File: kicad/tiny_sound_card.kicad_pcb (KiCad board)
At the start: 2 copper layers, 46 parts, among them CON1 BARREL_JACK, IC1 ATMEGA328P-A, J1 TRS_JACK, M1 DFR0299, P1 EXT_PWR, P2 SPKOUT, P3 EXT_SW0, P4 EXT_I2C, P4 M3Drill, P5 EXT_SW1, P6 EXT_UART, P7 EXT_SPI/ISP, SW1 SlideSW, SW2 SW_PUSH, SW3 SW_PUSH, SW4 SW_PUSH, SW5 SlideSW, SW6 SW_PUSH, U1 STMPS2141S, Y1 16MHz

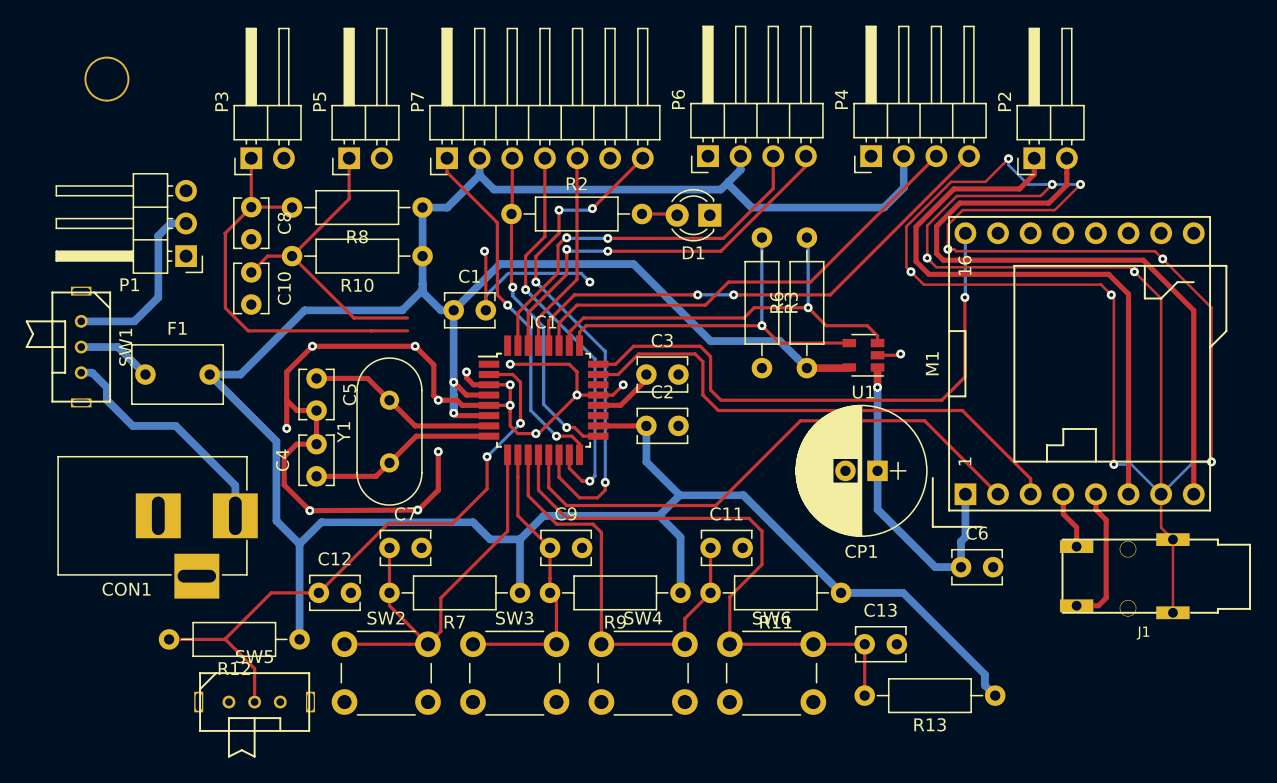
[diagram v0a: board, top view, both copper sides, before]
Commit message: 外形とパネル表裏を作成
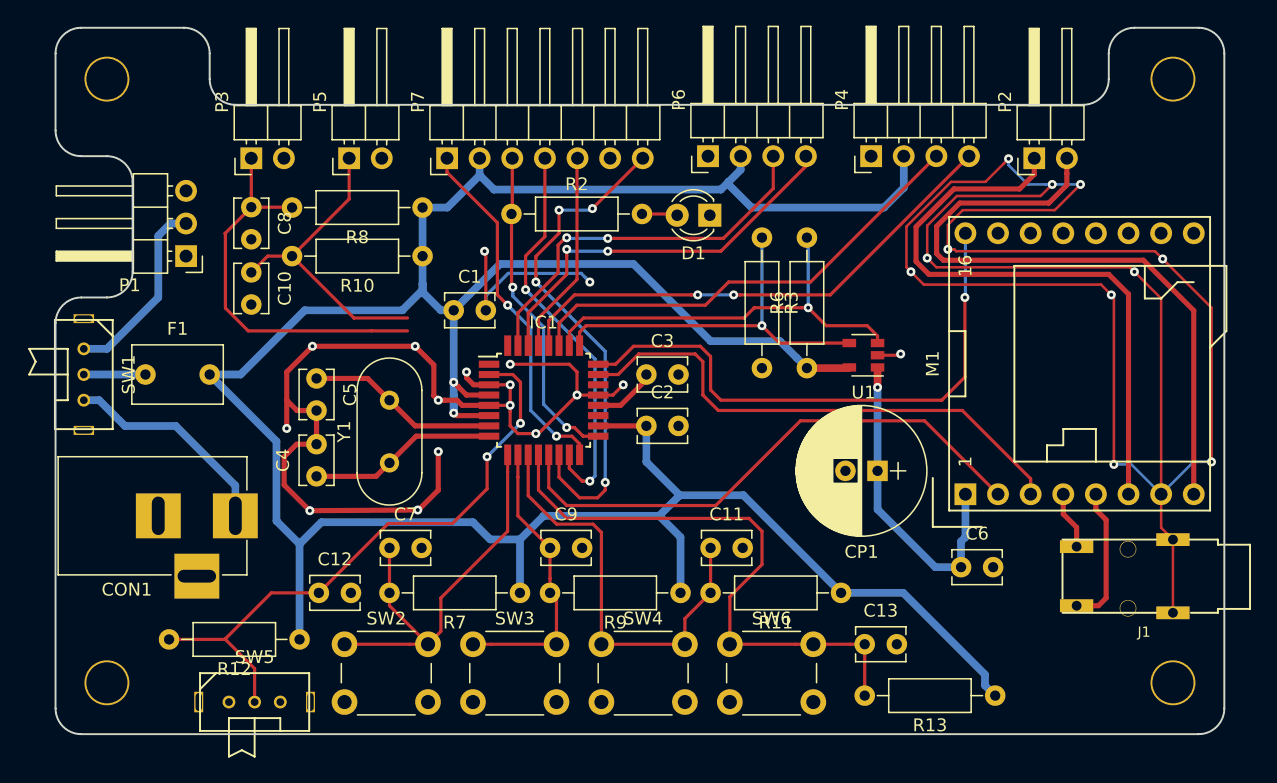
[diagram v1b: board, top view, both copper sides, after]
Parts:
- added P10: M3Drill, kamiya:M3Drill2, F.Cu at (138.0, 112.0)
- added P8: M3Drill, kamiya:M3Drill2, F.Cu at (55.0, 112.0)
- added P9: M3Drill, kamiya:M3Drill2, F.Cu at (138.0, 65.0)
- moved SW1 2.15 mm to (53.2, 88.0)
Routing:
- net /CONN_VCC: track 18.6 -> 16.9 mm
- net /SEL_VCC: track 5.89 -> 4.80 mm
- net /EXT_VCC: track 14.1 -> 14.8 mm
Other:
- board outline added: 91 x 55 mm
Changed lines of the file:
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@@
     (links 118)
     (no_connects 51)
-    (area 28.000002 48.15 144.375001 119.825)
+    (area 50.924999 60.924999 142.075001 116.075001)
     (thickness 1.6)
-    (drawings 14)
-    (tracks 483)
+    (drawings 62)
+    (tracks 480)
     (zones 0)
-    (modules 46)
+    (modules 49)
     (nets 47)
   )
@@
     (38 B.Mask user)
     (39 F.Mask user)
-    (40 Dwgs.User user)
+    (40 Dwgs.User user hide)
     (41 Cmts.User user)
     (42 Eco1.User user)
@@
     (add_net VCC)
   )
+  (module kamiya:M3Drill2 locked (layer F.Cu)
+    (at 138 112)
+    (fp_text reference P10 (at 0 3) (layer F.SilkS) hide
+      (effects (font (size 1 1) (thickness 0.15)))
+    )
+    (fp_text value M3Drill (at 0 -3) (layer F.Fab) hide
+      (effects (font (size 1 1) (thickness 0.15)))
+    )
+    (pad "" np_thru_hole circle (at 0 0) (size 3.5 3.5) (drill 3.2) (layers *.Cu F.SilkS)
+      (clearance 0.2))
+  )
+  (module kamiya:M3Drill2 locked (layer F.Cu)
+    (at 138 65)
+    (fp_text reference P9 (at 0 3) (layer F.SilkS) hide
+      (effects (font (size 1 1) (thickness 0.15)))
+    )
+    (fp_text value M3Drill (at 0 -3) (layer F.Fab) hide
+      (effects (font (size 1 1) (thickness 0.15)))
+    )
+    (pad "" np_thru_hole circle (at 0 0) (size 3.5 3.5) (drill 3.2) (layers *.Cu F.SilkS)
+      (clearance 0.2))
+  )
+  (module kamiya:M3Drill2 locked (layer F.Cu)
+    (at 55 112)
+    (fp_text reference P8 (at 0 3) (layer F.SilkS) hide
+      (effects (font (size 1 1) (thickness 0.15)))
+    )
+    (fp_text value M3Drill (at 0 -3) (layer F.Fab) hide
+      (effects (font (size 1 1) (thickness 0.15)))
+    )
+    (pad "" np_thru_hole circle (at 0 0) (size 3.5 3.5) (drill 3.2) (layers *.Cu F.SilkS)
+      (clearance 0.2))
+  )
   (module Capacitors_ThroughHole:C_Disc_D3.8mm_W2.6mm_P2.50mm (layer F.Cu)
     (at 82 83)
@@
   )
   (module kamiya:SK-12D01-VG4 (layer F.Cu)
-    (at 53 85.86 270)
+    (at 53.2 88 270)
     (descr http://akizukidenshi.com/catalog/g/gP-08789/)
     (tags SW)
@@
     )
   )
+  (gr_line (start 140 116) (end 53 116) (layer Eco2.User) (width 0.2))
+  (gr_line (start 142 63) (end 142 114) (layer Eco2.User) (width 0.2))
+  (gr_line (start 53 61) (end 140 61) (layer Eco2.User) (width 0.2))
+  (gr_line (start 51 114) (end 51 63) (layer Eco2.User) (width 0.2))
+  (gr_arc (start 53 114) (end 53 116) (angle 90) (layer Eco2.User) (width 0.2))
+  (gr_arc (start 140 114) (end 142 114) (angle 90) (layer Eco2.User) (width 0.2))
+  (gr_arc (start 140 63) (end 140 61) (angle 90) (layer Eco2.User) (width 0.2))
+  (gr_arc (start 53 63) (end 51 63) (angle 90) (layer Eco2.User) (width 0.2))
+  (gr_line (start 51 114) (end 51 63) (layer Eco1.User) (width 0.2))
+  (gr_line (start 70 116) (end 53 116) (layer Eco1.User) (width 0.2))
+  (gr_line (start 72 108) (end 72 114) (layer Eco1.User) (width 0.2))
+  (gr_line (start 110 106) (end 74 106) (layer Eco1.User) (width 0.2))
+  (gr_line (start 112 114) (end 112 108) (layer Eco1.User) (width 0.2))
+  (gr_line (start 140 116) (end 114 116) (layer Eco1.User) (width 0.2))
+  (gr_line (start 142 63) (end 142 114) (layer Eco1.User) (width 0.2))
+  (gr_line (start 53 61) (end 140 61) (layer Eco1.User) (width 0.2))
+  (gr_arc (start 53 114) (end 53 116) (angle 90) (layer Eco1.User) (width 0.2))
+  (gr_arc (start 70 114) (end 72 114) (angle 90) (layer Eco1.User) (width 0.2))
+  (gr_arc (start 74 108) (end 72 108) (angle 90) (layer Eco1.User) (width 0.2))
+  (gr_arc (start 110 108) (end 110 106) (angle 90) (layer Eco1.User) (width 0.2))
+  (gr_arc (start 114 114) (end 114 116) (angle 90) (layer Eco1.User) (width 0.2))
+  (gr_arc (start 140 114) (end 142 114) (angle 90) (layer Eco1.User) (width 0.2))
+  (gr_arc (start 140 63) (end 140 61) (angle 90) (layer Eco1.User) (width 0.2))
+  (gr_arc (start 53 63) (end 51 63) (angle 90) (layer Eco1.User) (width 0.2))
+  (gr_line (start 51 69) (end 51 63) (layer Edge.Cuts) (width 0.15))
+  (gr_line (start 55 71) (end 53 71) (layer Edge.Cuts) (width 0.15))
+  (gr_line (start 57 80) (end 57 73) (layer Edge.Cuts) (width 0.15))
+  (gr_arc (start 53 69) (end 53 71) (angle 90) (layer Edge.Cuts) (width 0.15))
+  (gr_arc (start 55 73) (end 55 71) (angle 90) (layer Edge.Cuts) (width 0.15))
+  (gr_line (start 53 82) (end 55 82) (layer Edge.Cuts) (width 0.15))
+  (gr_line (start 51 114) (end 51 84) (layer Edge.Cuts) (width 0.15))
+  (gr_line (start 140 116) (end 53 116) (layer Edge.Cuts) (width 0.15))
+  (gr_line (start 142 63) (end 142 114) (layer Edge.Cuts) (width 0.15))
+  (gr_line (start 135 61) (end 140 61) (layer Edge.Cuts) (width 0.15))
+  (gr_line (start 133 65) (end 133 63) (layer Edge.Cuts) (width 0.15))
+  (gr_line (start 65 67) (end 131 67) (layer Edge.Cuts) (width 0.15))
+  (gr_line (start 63 63) (end 63 65) (layer Edge.Cuts) (width 0.15))
+  (gr_line (start 61 61) (end 53 61) (layer Edge.Cuts) (width 0.15))
+  (gr_arc (start 53 84) (end 51 84) (angle 90) (layer Edge.Cuts) (width 0.15))
+  (gr_arc (start 55 80) (end 57 80) (angle 90) (layer Edge.Cuts) (width 0.15))
+  (gr_arc (start 53 114) (end 53 116) (angle 90) (layer Edge.Cuts) (width 0.15))
+  (gr_arc (start 140 114) (end 142 114) (angle 90) (layer Edge.Cuts) (width 0.15))
+  (gr_arc (start 140 63) (end 140 61) (angle 90) (layer Edge.Cuts) (width 0.15))
+  (gr_arc (start 135 63) (end 133 63) (angle 90) (layer Edge.Cuts) (width 0.15))
+  (gr_arc (start 65 65) (end 65 67) (angle 90) (layer Edge.Cuts) (width 0.15))
+  (gr_arc (start 131 65) (end 133 65) (angle 90) (layer Edge.Cuts) (width 0.15))
+  (gr_arc (start 61 63) (end 61 61) (angle 90) (layer Edge.Cuts) (width 0.15))
+  (gr_arc (start 53 63) (end 51 63) (angle 90) (layer Edge.Cuts) (width 0.15))
   (gr_line (start 134 108) (end 142 108) (layer Dwgs.User) (width 0.2))
   (gr_line (start 134 116) (end 134 108) (layer Dwgs.User) (width 0.2))
@@
   (segment (start 121.84 100.66) (end 121.84 97.32) (width 0.6) (layer B.Cu) (net 32))
   (segment (start 121.5 103) (end 121.5 101) (width 0.6) (layer B.Cu) (net 32))
-  (segment (start 55 89) (end 53.86 87.86) (width 0.6) (layer B.Cu) (net 33))
-  (segment (start 53.86 87.86) (end 53 87.86) (width 0.6) (layer B.Cu) (net 33))
-  (segment (start 55 90) (end 55 89) (width 0.6) (layer B.Cu) (net 33))
-  (segment (start 57 92) (end 55 90) (width 0.6) (layer B.Cu) (net 33))
-  (segment (start 60.35 92) (end 57 92) (width 0.6) (layer B.Cu) (net 33))
   (segment (start 65 99) (end 65 96.65) (width 0.6) (layer B.Cu) (net 33))
   (segment (start 65 96.65) (end 60.35 92) (width 0.6) (layer B.Cu) (net 33))
-  (segment (start 53 85.86) (end 55.86 85.86) (width 0.6) (layer B.Cu) (net 34))
-  (segment (start 55.86 85.86) (end 58 88) (width 0.6) (layer B.Cu) (net 34))
+  (segment (start 60.35 92) (end 56.4 92) (width 0.6) (layer B.Cu) (net 33))
+  (segment (start 56.4 92) (end 54.4 90) (width 0.6) (layer B.Cu) (net 33))
+  (segment (start 54.4 90) (end 53.2 90) (width 0.6) (layer B.Cu) (net 33))
+  (segment (start 53.2 88) (end 58 88) (width 0.6) (layer B.Cu) (net 34))
   (segment (start 61.16 76.24) (end 59.957919 76.24) (width 0.6) (layer B.Cu) (net 35))
   (segment (start 59.957919 76.24) (end 59 77.197919) (width 0.6) (layer B.Cu) (net 35))
   (segment (start 59 77.197919) (end 59 82) (width 0.6) (layer B.Cu) (net 35))
-  (segment (start 59 82) (end 57.14 83.86) (width 0.6) (layer B.Cu) (net 35))
-  (segment (start 57.14 83.86) (end 53 83.86) (width 0.6) (layer B.Cu) (net 35))
+  (segment (start 55 86) (end 53.2 86) (width 0.6) (layer B.Cu) (net 35))
+  (segment (start 59 82) (end 55 86) (width 0.6) (layer B.Cu) (net 35))
   (segment (start 132 97.32) (end 132 98.522081) (width 0.4) (layer F.Cu) (net 36))
   (segment (start 132 98.522081) (end 132.8 99.322081) (width 0.4) (layer F.Cu) (net 36))
